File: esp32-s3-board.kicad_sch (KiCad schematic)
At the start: 5 parts, among them P1 USB_C_Plug_USB2.0, U1 ESP32-S3, U2 AMS1117-3.3

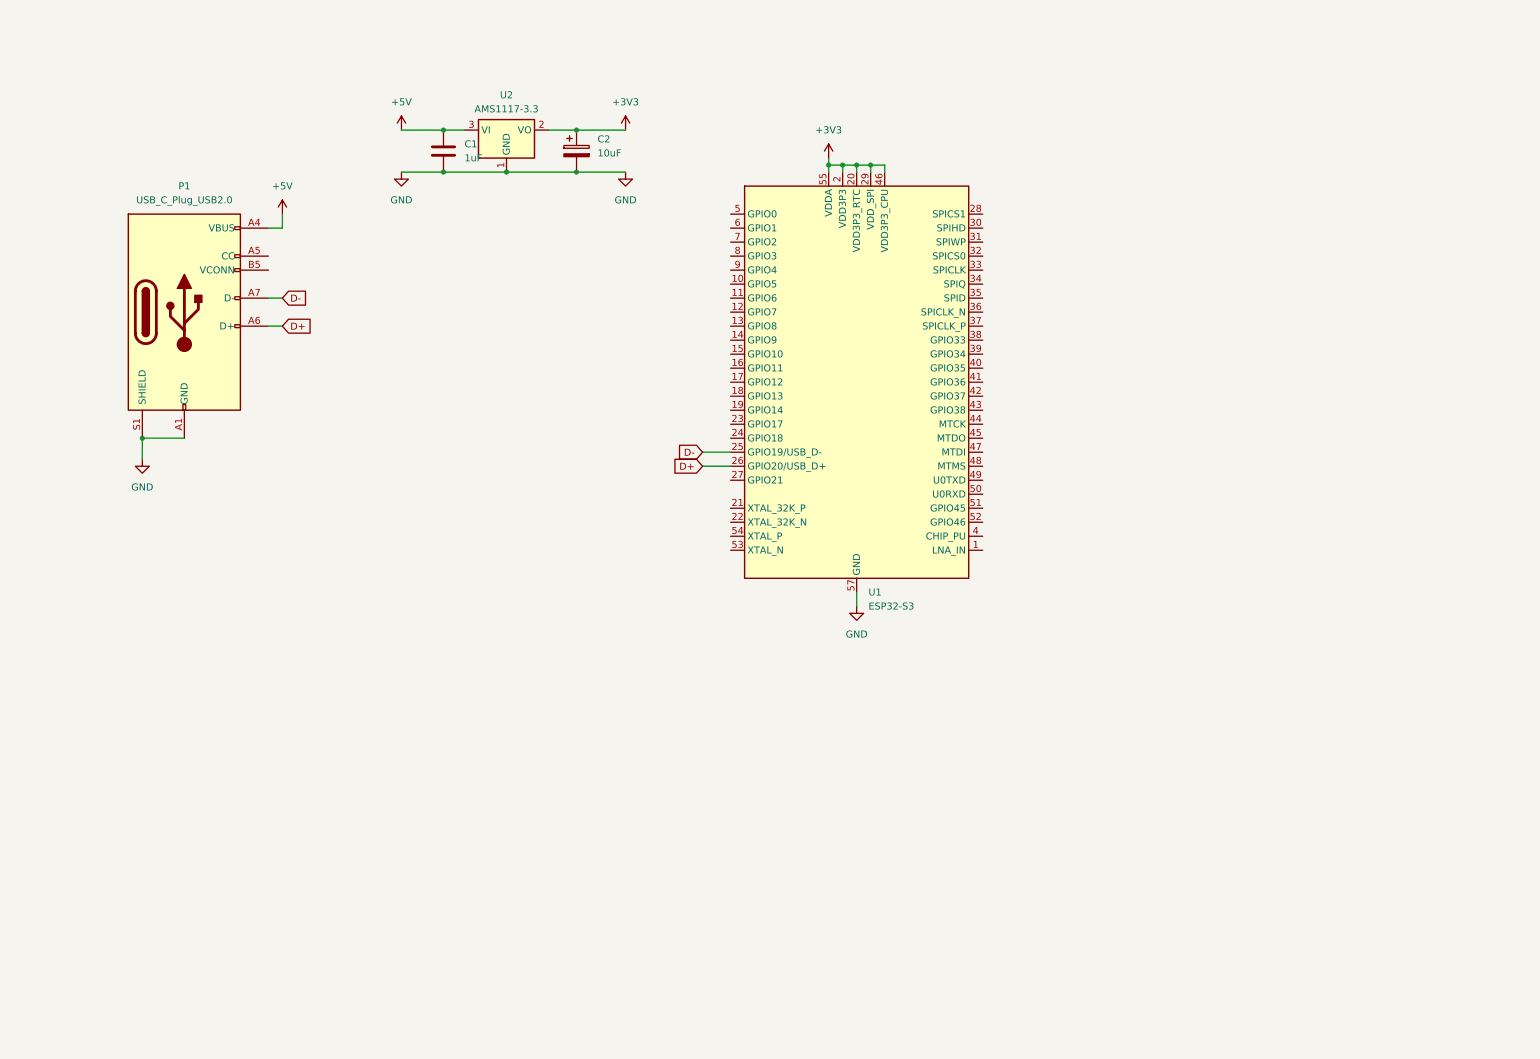
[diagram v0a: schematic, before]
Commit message: Added journal
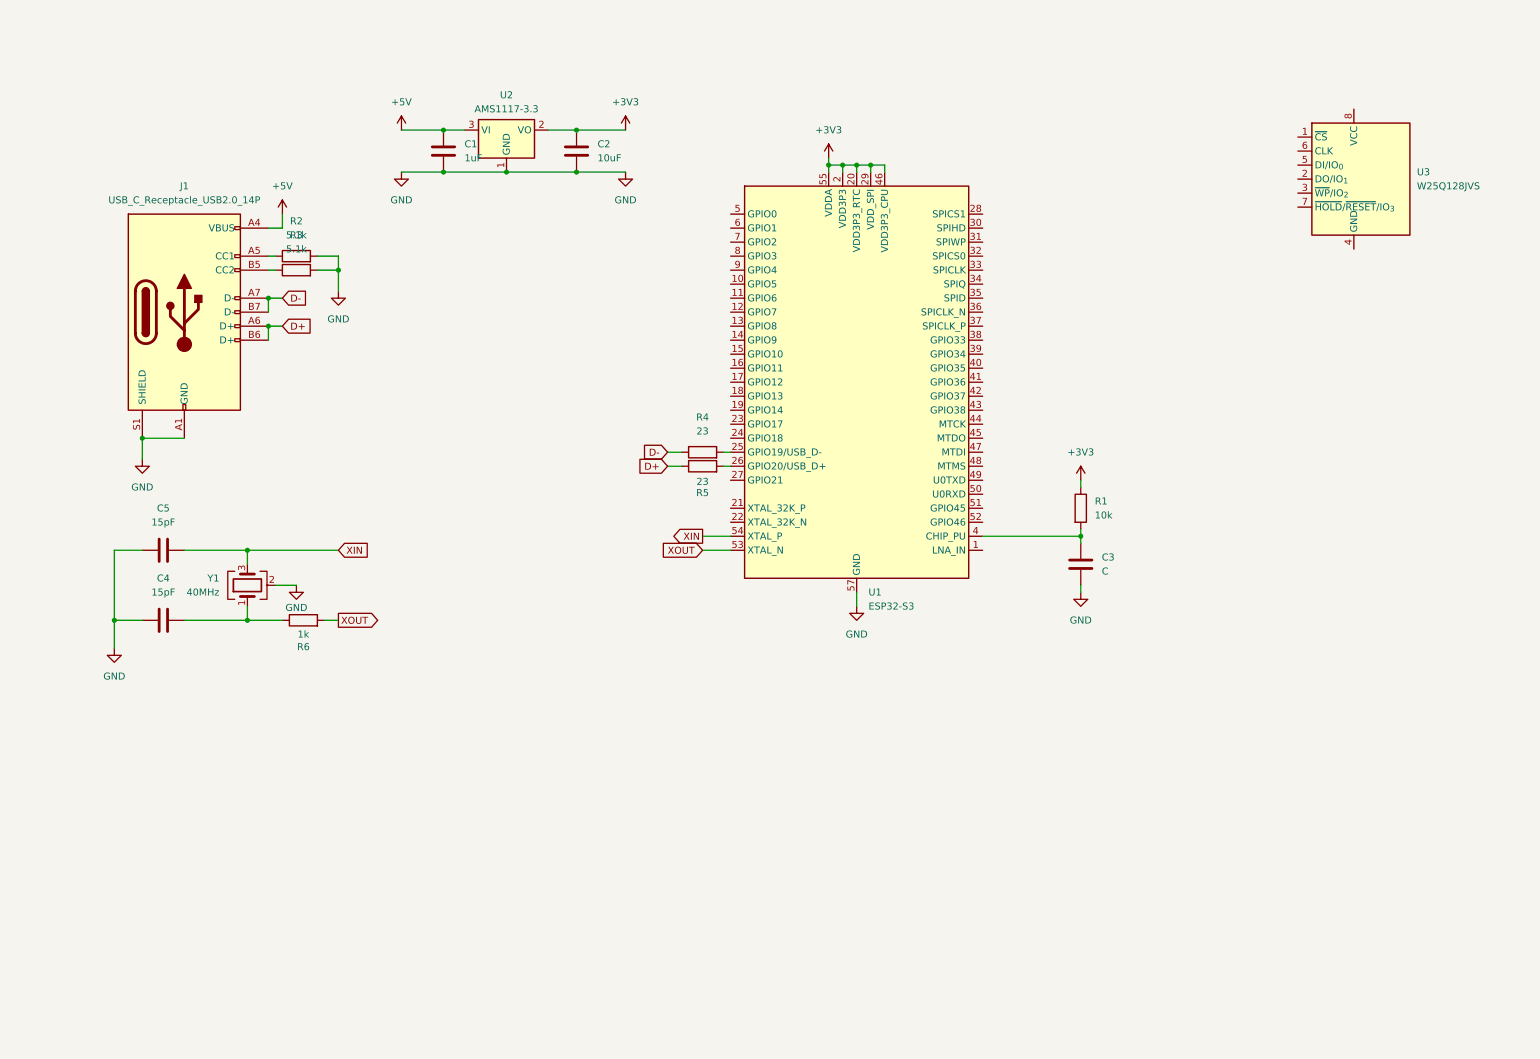
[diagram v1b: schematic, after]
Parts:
- removed C2: 10uF, symbol Device:C_Polarized
- removed P1: USB_C_Plug_USB2.0, symbol Connector:USB_C_Plug_USB2.0
- added C2: 10uF, symbol Device:C
- added C3: C, symbol Device:C
- added C4, C5: 15pF, symbol Device:C
- added J1: USB_C_Receptacle_USB2.0_14P, symbol Connector:USB_C_Receptacle_USB2.0_14P
- added R1: 10k, symbol Device:R
- added R2, R3: 5.1k, symbol Device:R
- added R4, R5: 23, symbol Device:R
- added R6: 1k, symbol Device:R
- added U3: W25Q128JVS, Package_SO:SOIC-8_5.3x5.3mm_P1.27mm, symbol Memory_Flash:W25Q128JVS
- added Y1: 40MHz, symbol Device:Crystal_GND24
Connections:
- net +3V3: now also C2.1, R1.1
- net +5V: now also J1.A4 (VBUS), J1.A9 (VBUS), J1.B4 (VBUS), J1.B9 (VBUS)
- net D+: now also J1.A6 (D+), J1.B6 (D+), R5.1; no longer U1.26 (GPIO20/USB_D+)
- net D-: now also J1.A7 (D-), J1.B7 (D-), R4.1; no longer U1.25 (GPIO19/USB_D-)
- net GND: now also C2.2, C3.2, C4.1, C5.1, J1.A1 (GND), J1.A12 (GND), J1.B1 (GND), J1.B12 (GND), J1.S1 (SHIELD), R2.2, R3.2, Y1.2 (G), Y1.4 (G)
- net at U1.4 (CHIP_PU): now also C3.1, R1.2
- net XOUT: now reaches U1.53 (XTAL_N)
- net XOUT: now also R6.2
- net XIN: now reaches U1.54 (XTAL_P)
- net XIN: now also C5.2, Y1.3
- new net: R4.2, U1.25 (GPIO19/USB_D-)
- new net: R5.2, U1.26 (GPIO20/USB_D+)
- new net: C4.2, R6.1, Y1.1
- new net: J1.A5 (CC1), R2.1
- new net: J1.B5 (CC2), R3.1

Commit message: Editted journal
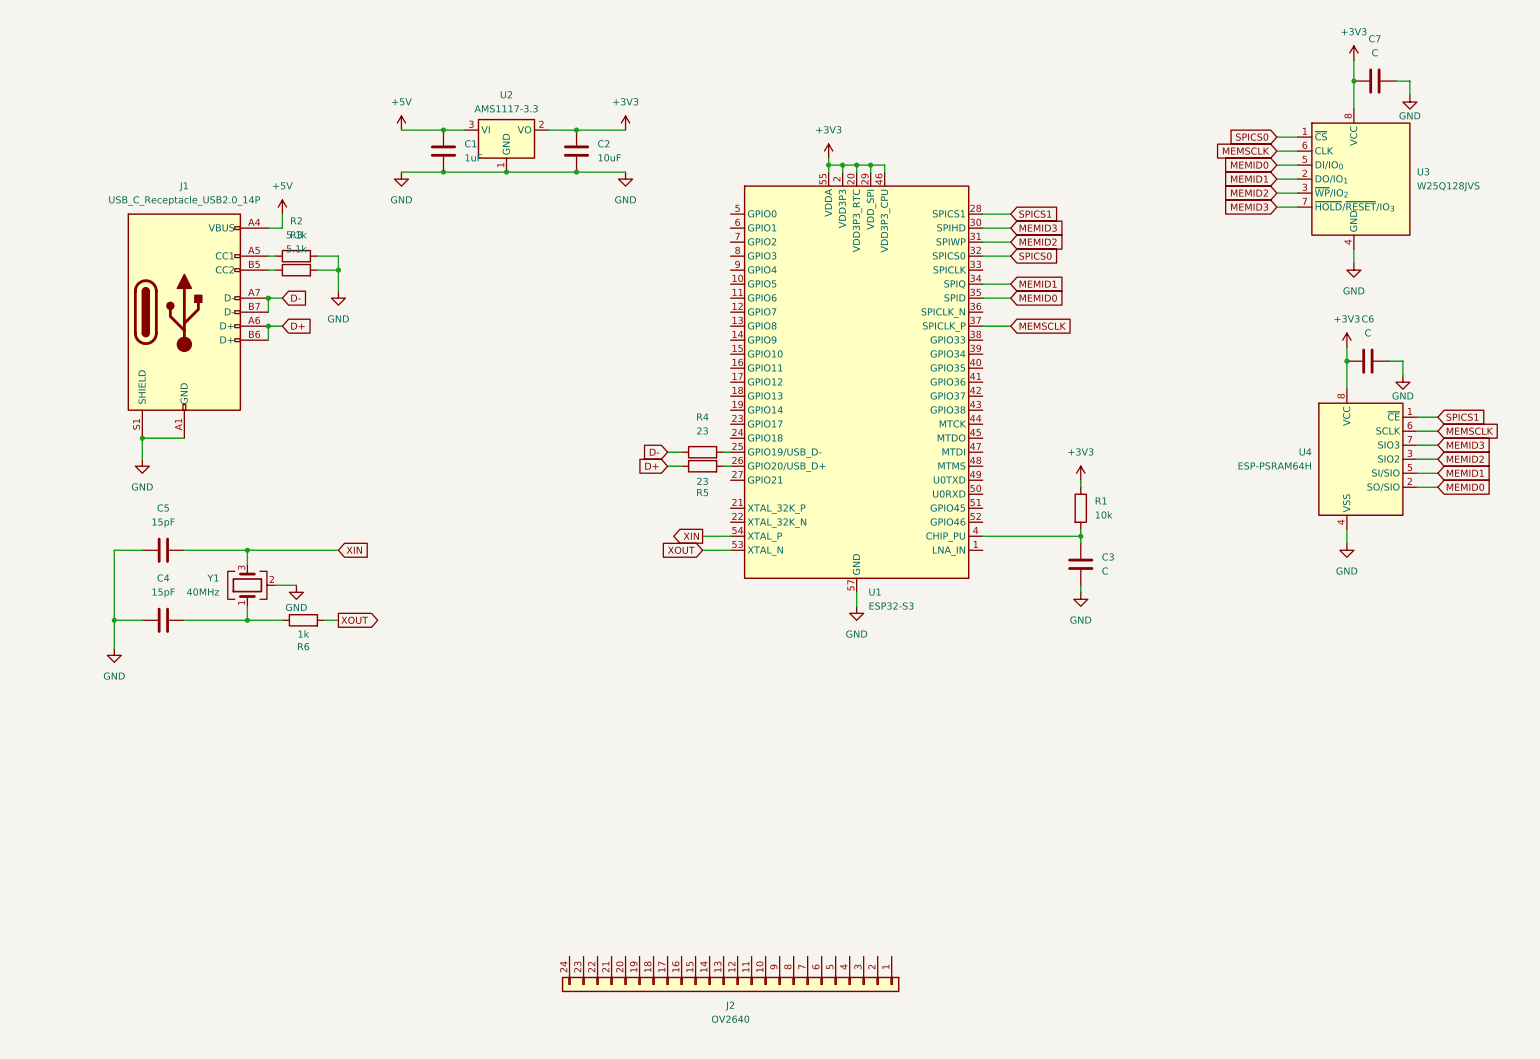
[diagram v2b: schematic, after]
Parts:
- added C6, C7: C, symbol Device:C
- added J2: OV2640, symbol Connector_Generic:Conn_01x24
- added U4: ESP-PSRAM64H, Package_SO:SOIC-8_3.9x4.9mm_P1.27mm, symbol Memory_RAM:ESP-PSRAM32
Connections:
- net +3V3: now also U3.8 (VCC), C6.1, C7.1, U4.8 (VCC)
- net GND: now also U3.4 (GND), C6.2, C7.2, U4.4 (VSS)
- net SPICS1: now reaches U1.28 (SPICS1)
- net SPICS1: now also U4.1 (~{CE})
- net MEMID3: now reaches U1.30 (SPIHD)
- net MEMID3: now also U3.7 (~{HOLD}/~{RESET}/IO_{3}), U4.7 (SIO3)
- net MEMID2: now reaches U1.31 (SPIWP)
- net MEMID2: now also U3.3 (~{WP}/IO_{2}), U4.3 (SIO2)
- net SPICS0: now reaches U1.32 (SPICS0)
- net SPICS0: now also U3.1 (~{CS})
- net MEMID1: now reaches U1.34 (SPIQ)
- net MEMID1: now also U3.2 (DO/IO_{1}), U4.5 (SI/SIO)
- net MEMID0: now reaches U1.35 (SPID)
- net MEMID0: now also U3.5 (DI/IO_{0}), U4.2 (SO/SIO)
- net MEMSCLK: now reaches U1.37 (SPICLK_P)
- net MEMSCLK: now also U3.6 (CLK), U4.6 (SCLK)

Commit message: Added journal
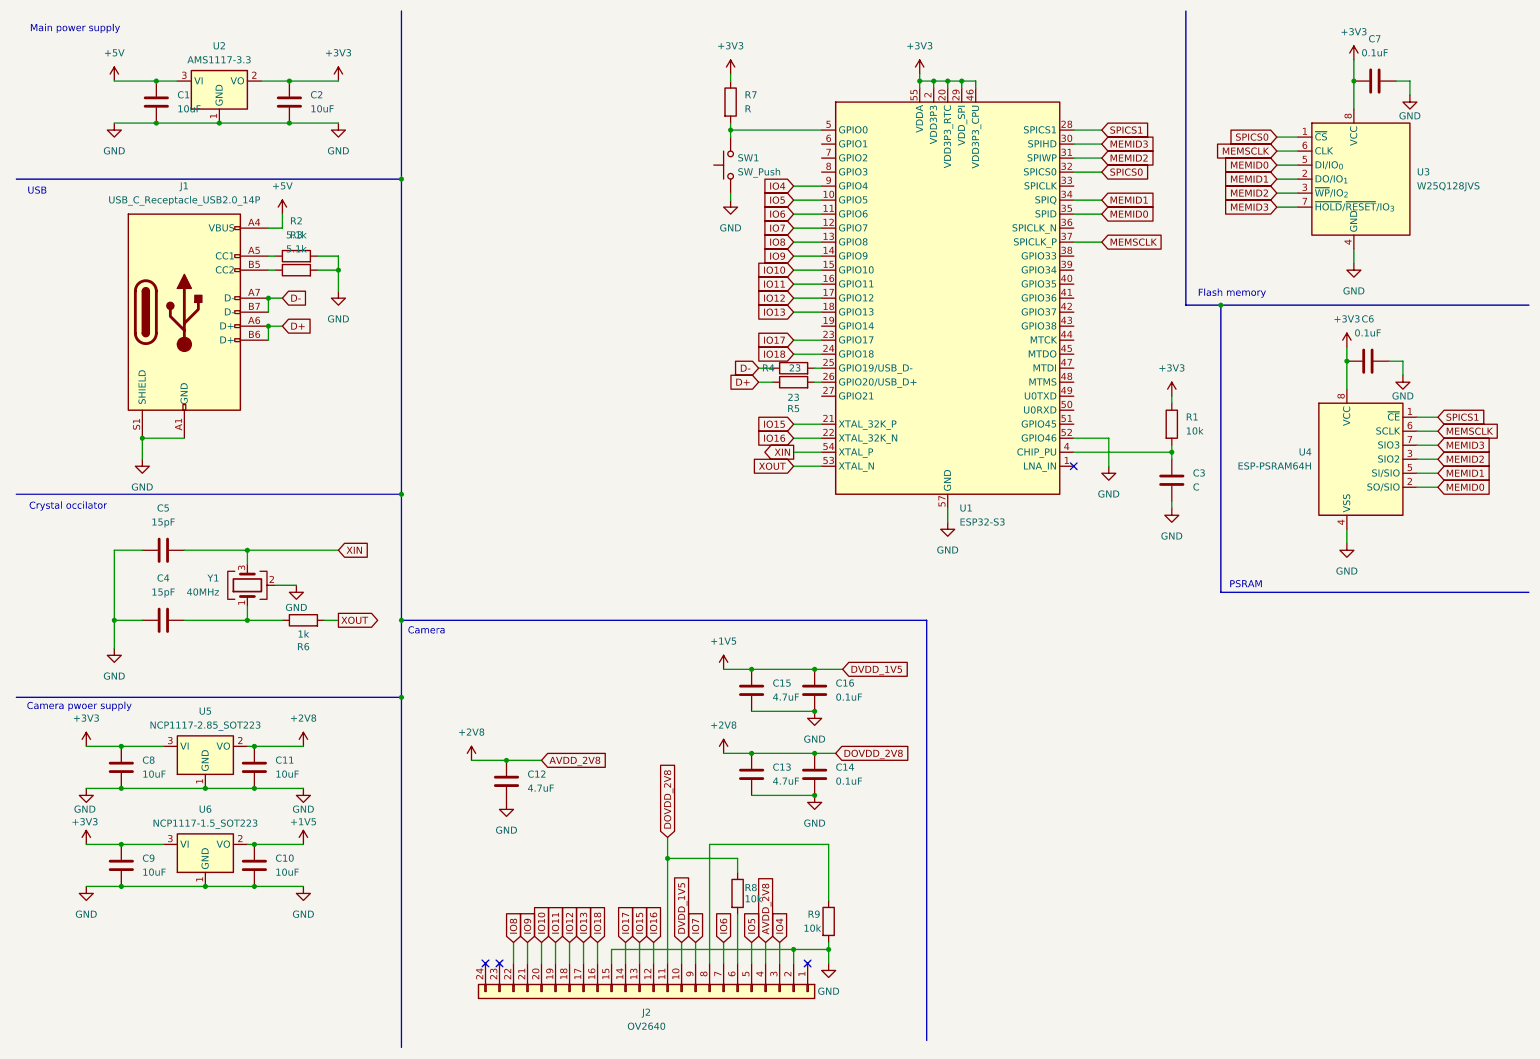
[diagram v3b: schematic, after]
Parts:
- added C10, C11, C8, C9: 10uF, symbol Device:C
- added C12, C13, C15: 4.7uF, symbol Device:C
- added C14, C16: 0.1uF, symbol Device:C
- added R7: R, symbol Device:R
- added R8, R9: 10k, symbol Device:R
- added SW1: SW_Push, symbol Switch:SW_Push
- added U5: NCP1117-2.85_SOT223, Package_TO_SOT_SMD:SOT-223-3_TabPin2, symbol Regulator_Linear:NCP1117-2.85_SOT223
- added U6: NCP1117-1.5_SOT223, Package_TO_SOT_SMD:SOT-223-3_TabPin2, symbol Regulator_Linear:NCP1117-1.5_SOT223
- C1: value 1uF -> 10uF
- C6, C7: value C -> 0.1uF
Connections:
- net +3V3: now also C8.1, C9.1, R7.1, U5.3 (VI), U6.3 (VI)
- net GND: now also J2.15 (Pin_15), J2.2 (Pin_2), U1.52 (GPIO46), C10.2, C11.2, C12.2, C13.2, C14.2, C15.2, C16.2, C8.2, C9.2, R9.2, SW1.1, U5.1 (GND), U6.1 (GND)
- net IO5: now reaches U1.10 (GPIO5)
- net IO5: now also J2.5 (Pin_5)
- net IO6: now reaches U1.11 (GPIO6)
- net IO6: now also J2.7 (Pin_7)
- net IO7: now reaches U1.12 (GPIO7)
- net IO7: now also J2.9 (Pin_9)
- net IO8: now reaches U1.13 (GPIO8)
- net IO8: now also J2.22 (Pin_22)
- net IO9: now reaches U1.14 (GPIO9)
- net IO9: now also J2.21 (Pin_21)
- net IO10: now reaches U1.15 (GPIO10)
- net IO10: now also J2.20 (Pin_20)
- net IO11: now reaches U1.16 (GPIO11)
- net IO11: now also J2.19 (Pin_19)
- net IO12: now reaches U1.17 (GPIO12)
- net IO12: now also J2.18 (Pin_18)
- net IO13: now reaches U1.18 (GPIO13)
- net IO13: now also J2.17 (Pin_17)
- net IO15: now reaches U1.21 (XTAL_32K_P)
- net IO15: now also J2.13 (Pin_13)
- net IO16: now reaches U1.22 (XTAL_32K_N)
- net IO16: now also J2.12 (Pin_12)
- net IO17: now reaches U1.23 (GPIO17)
- net IO17: now also J2.14 (Pin_14)
- net IO18: now reaches U1.24 (GPIO18)
- net IO18: now also J2.16 (Pin_16)
- net at U1.5 (GPIO0): now also R7.2, SW1.2
- net IO4: now reaches U1.9 (GPIO4)
- net IO4: now also J2.3 (Pin_3)
- net +1V5: now reaches J2.10 (Pin_10)
- net +1V5: now also C10.1, C15.1, C16.1, U6.2 (VO)
- net +2V8: now reaches J2.11 (Pin_11)
- net +2V8: now also J2.4 (Pin_4), C11.1, C12.1, C13.1, C14.1, R8.1, U5.2 (VO)
- net at J2.6 (Pin_6): now also R8.2
- net at J2.8 (Pin_8): now also R9.1
- no-connect marks 0 -> 4
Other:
- note added: "Camera"
- note added: "Camera pwoer supply"
- note added: "Crystal occilator"
- note added: "Flash memory"
- note added: "Main power supply"
- note added: "PSRAM"
- note added: "USB"
- moved on the sheet: C1, C2, C3, J2, R1, R4, R5, U1, U2
